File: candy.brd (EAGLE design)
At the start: 26 x 26 mm, 8 parts

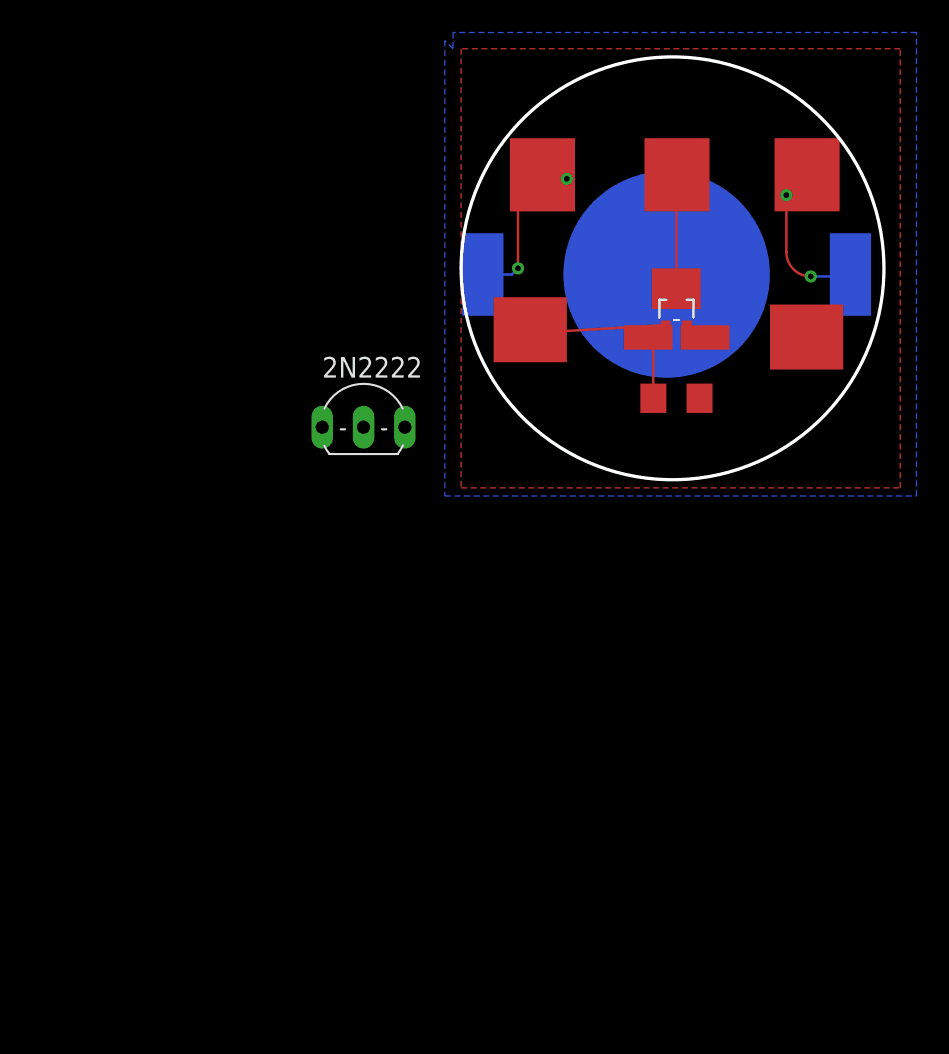
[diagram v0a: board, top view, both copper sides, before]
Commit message: board ready for silk
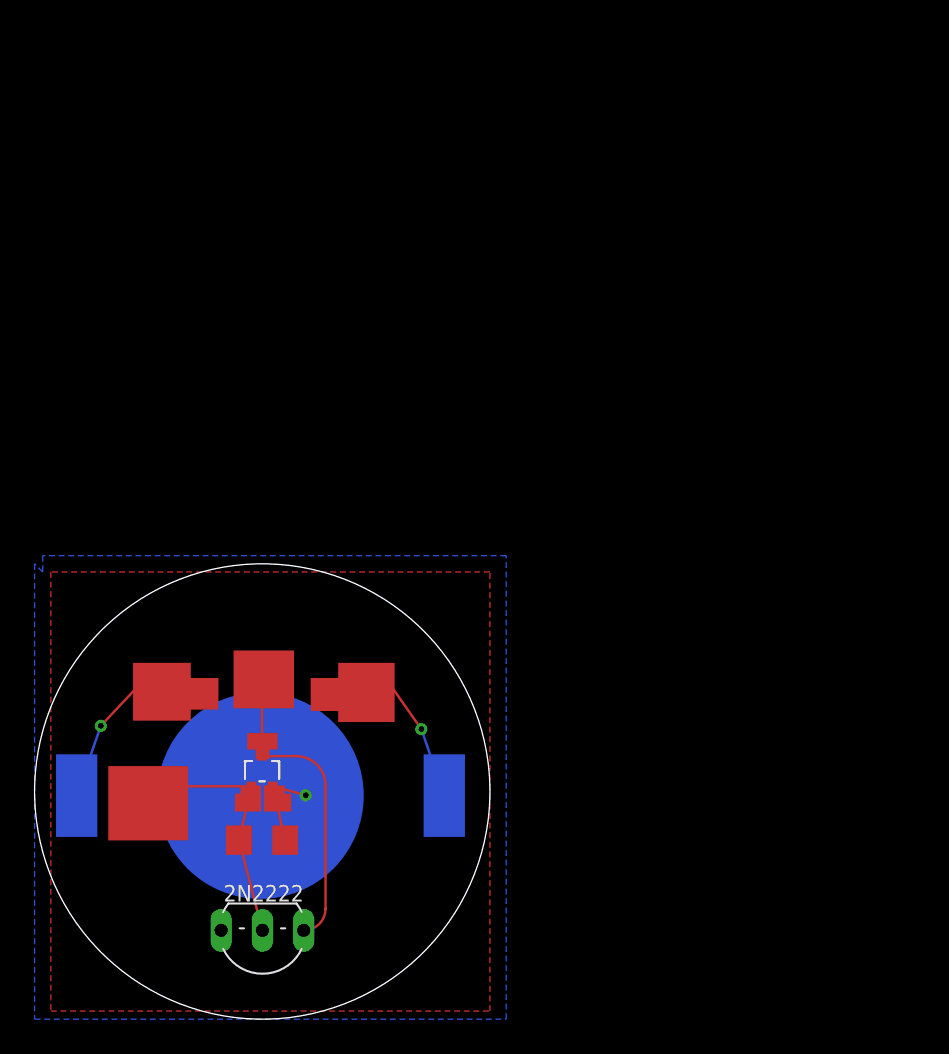
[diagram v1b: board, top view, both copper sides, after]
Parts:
- 2N2222: device transistor-neu-to92:TO92-EBC -> TinyTony_ShenzenReady:TO92-EBC
- moved U$4 41.0 mm to (12.8, 18.8)
- moved U$7 40.6 mm to (12.7, 12.6)
- moved U$5 40.5 mm to (20.3, 19.8)
- moved VCC 39.2 mm to (5.53, 19.7)
- moved N-MOSFET 38.1 mm to (12.8, 14.1)
- moved 10M 37.3 mm to (12.8, 9.83)
- moved U$1 35.3 mm to (7.47, 13.2)
- moved 2N2222 34.1 mm to (12.8, 3.02), turned to 180 degrees
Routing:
- net LOAD: track 7.50 -> 17.9 mm
- net GND: track 0.00 -> 5.52 mm, vias 0 -> 1
- net VCC: track 20.5 -> 16.6 mm, vias 4 -> 2
- net N$1: track 13.1 -> 13.8 mm
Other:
- board size 26 x 26 mm -> 28 x 28 mm
- board text added: "G:/_GIT/candy/artwork.bmp"

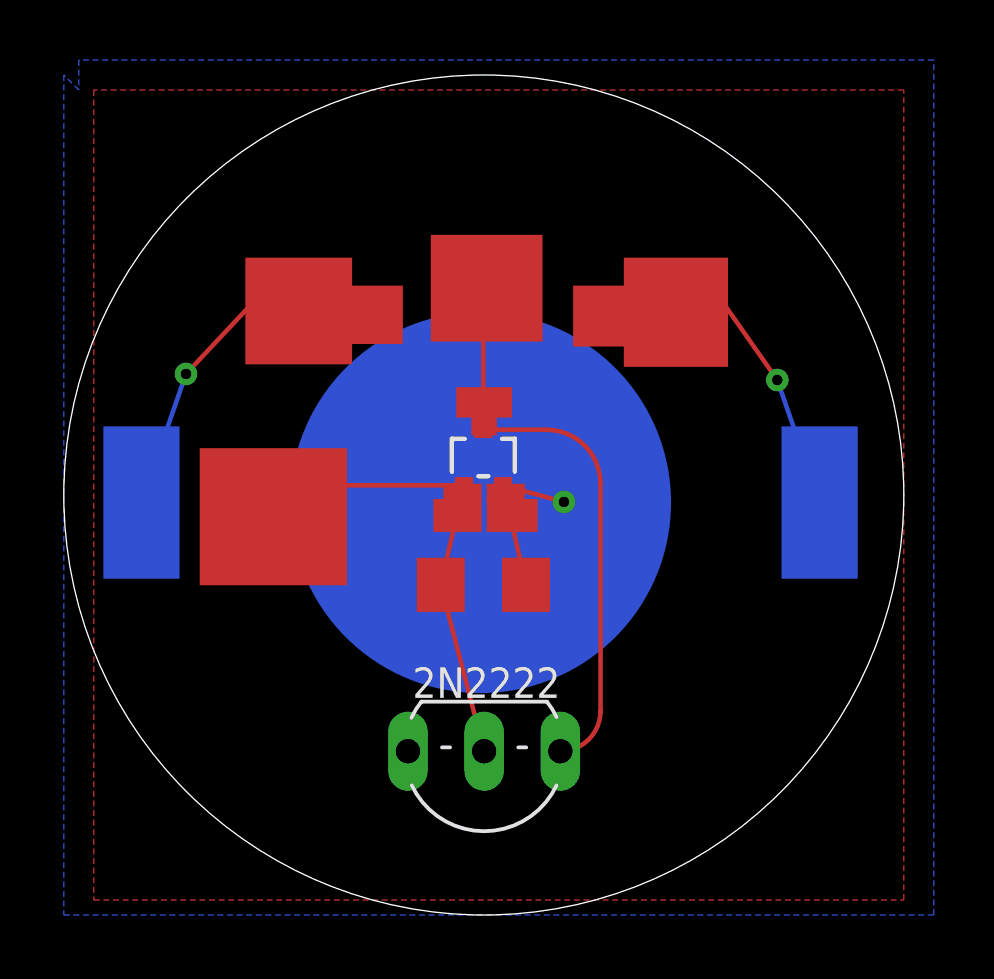
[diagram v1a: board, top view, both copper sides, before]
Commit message: shifted a bit
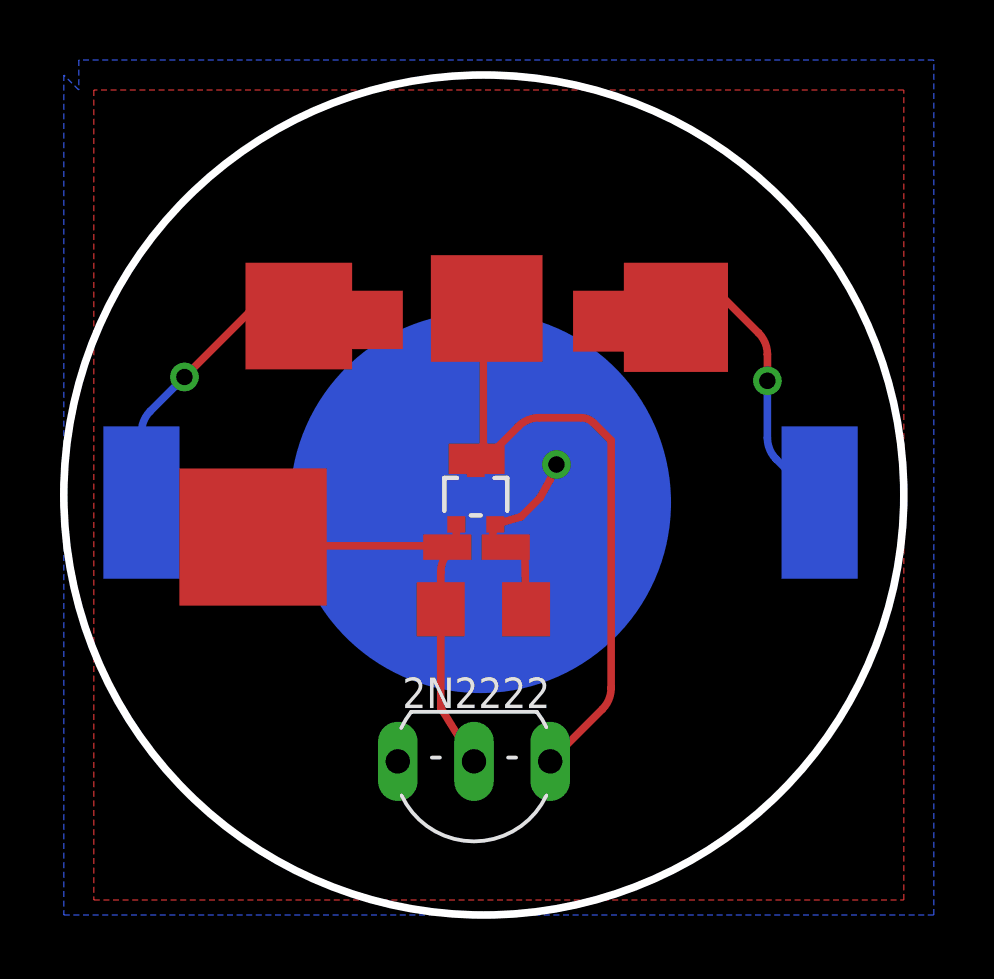
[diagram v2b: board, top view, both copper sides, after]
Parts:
- moved U$1 2.17 mm to (6.71, 11.1)
- moved N-MOSFET 1.33 mm to (12.5, 12.8)
- moved VCC 0.94 mm to (5.62, 18.8)
- moved 10M 0.81 mm to (12.8, 9.02)
- moved U$4 0.68 mm to (12.8, 18.1)
- moved 2N2222 0.48 mm to (12.4, 2.68)
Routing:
- net GND: track 5.52 -> 10.9 mm
- net LOAD: track 17.9 -> 21.5 mm
- net VCC: track 16.6 -> 17.6 mm
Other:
- board text added: "G:/_GIT/candy/gfx/artwork-draw.bmp"
